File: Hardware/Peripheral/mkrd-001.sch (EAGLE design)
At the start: 5 parts, among them J1 MKR

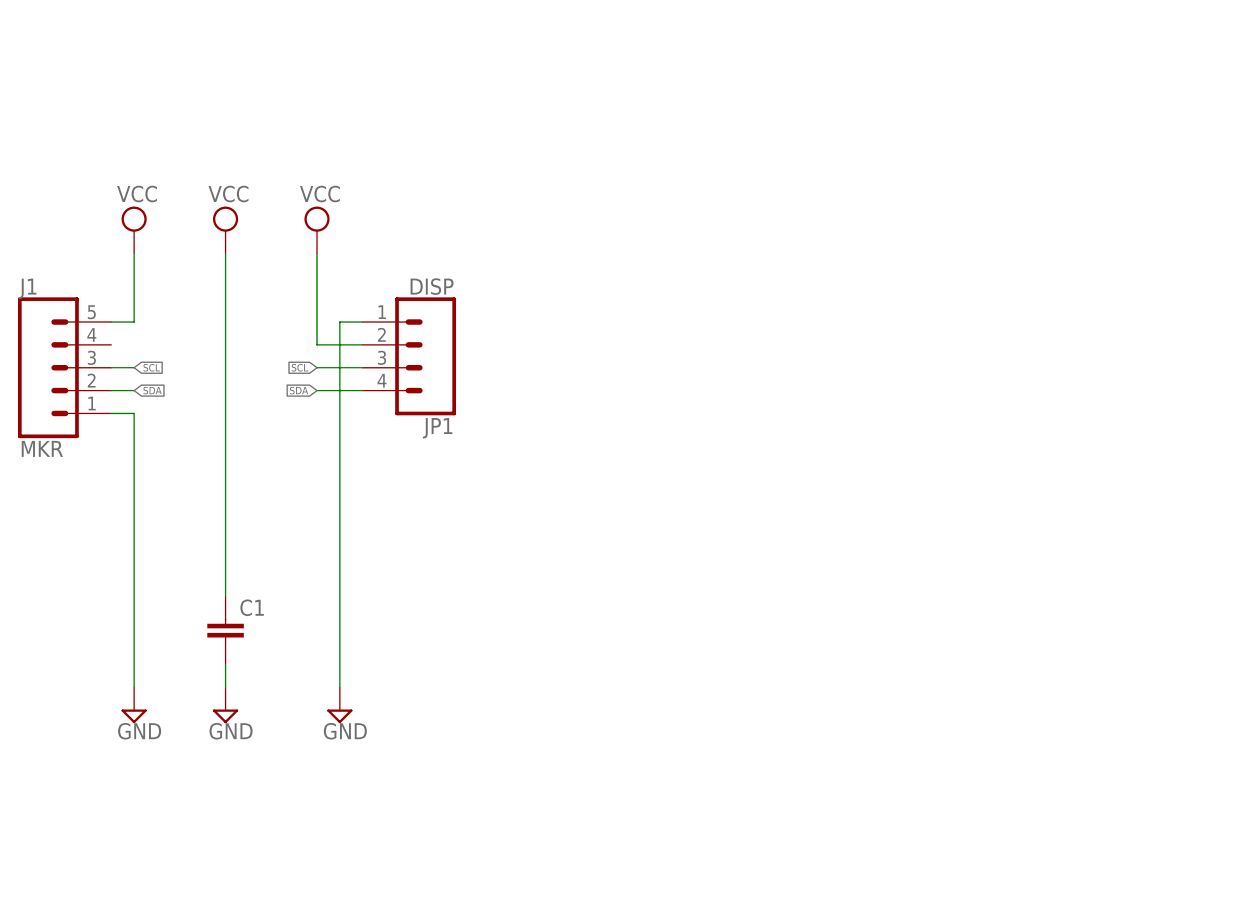
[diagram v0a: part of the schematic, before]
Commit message: Added new board.
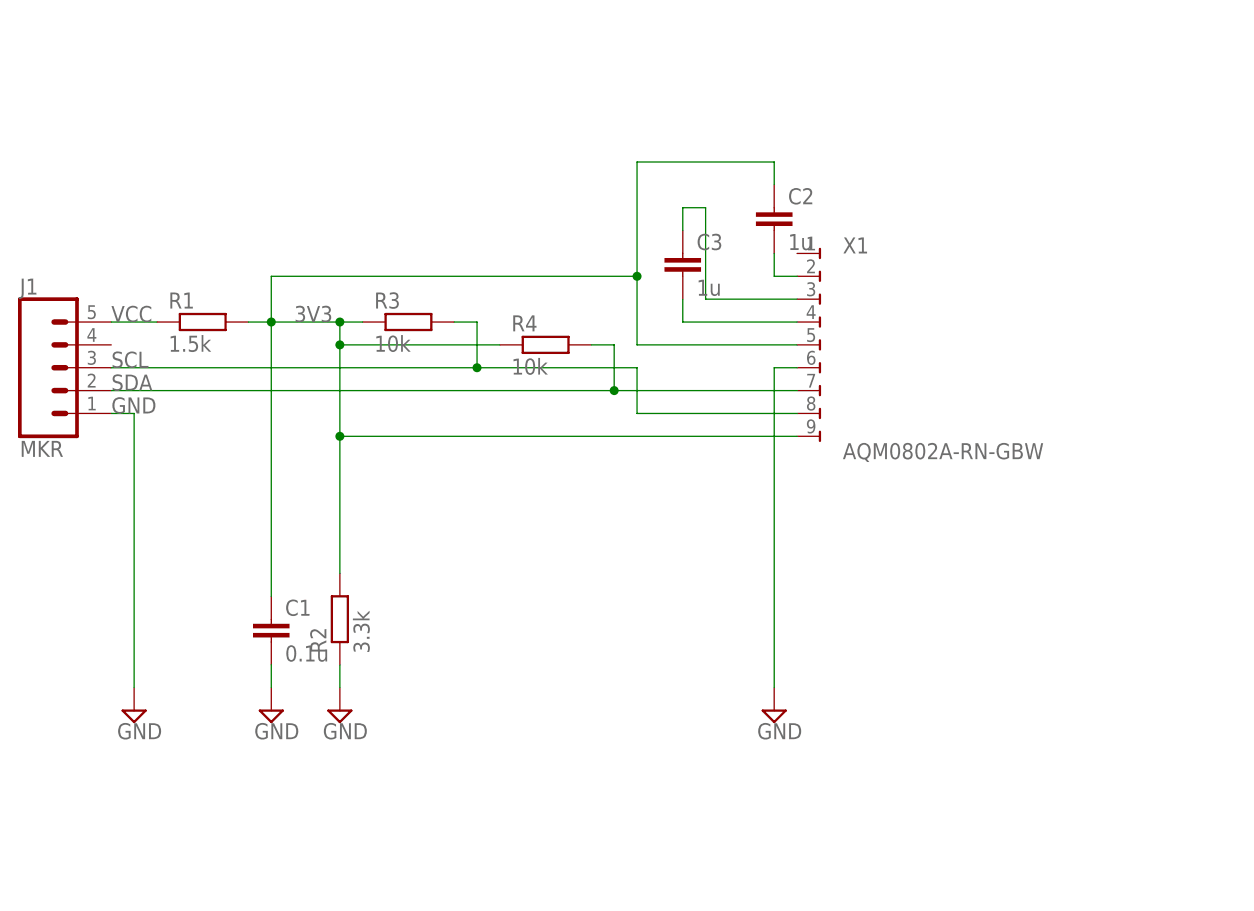
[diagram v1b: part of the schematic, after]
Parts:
- removed JP1: DISP, SparkFun-Connectors:CONN_04
- added C2, C3: 1u, rcl:C-EU025-025X050
- added R1: 1.5k, rcl:R-EU_0204/5
- added R2: 3.3k, rcl:R-EU_0204/5
- added R3, R4: 10k, rcl:R-EU_0204/5
- added X1: AQM0802A-RN-GBW, AQM0802A-RN-GBW:AQM0802A-RN-GBW
- C1: value (none) -> 0.1u
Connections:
- new net 3V3: C1.1, C2.1, R1.2, R2.2, R3.1, R4.1, X1.5, X1.9
- new net N$1: C2.2, X1.2
- new net N$2: C3.2, X1.4
- new net N$3: C3.1, X1.3
- net GND: now also R2.1, X1.6; no longer JP1.1
- net SCL: now also R3.2, X1.8; no longer JP1.3
- net SDA: now also R4.2, X1.7; no longer JP1.4
- net VCC: now also R1.1; no longer C1.1, JP1.2
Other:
- moved on the sheet: C1

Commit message: Signal name.
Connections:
- net N$1 renamed LCDVOUT
- net N$2 renamed CAP1P
- net N$3 renamed CAP1N
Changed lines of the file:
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@@
 </segment>
 </net>
-<net name="N$2" class="0">
+<net name="CAP1P" class="0">
 <segment>
 <pinref part="X1" gate="G$1" pin="4"/>
@@
 </segment>
 </net>
-<net name="N$3" class="0">
+<net name="CAP1N" class="0">
 <segment>
 <pinref part="C3" gate="G$1" pin="1"/>
@@
 </segment>
 </net>
-<net name="N$1" class="0">
+<net name="LCDVOUT" class="0">
 <segment>
 <pinref part="X1" gate="G$1" pin="2"/>
